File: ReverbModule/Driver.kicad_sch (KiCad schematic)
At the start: 29 parts, among them J1 Tank, J2 Screw_Terminal_01x02, Q1 BD139, Q2 BD140, U1 NE5532

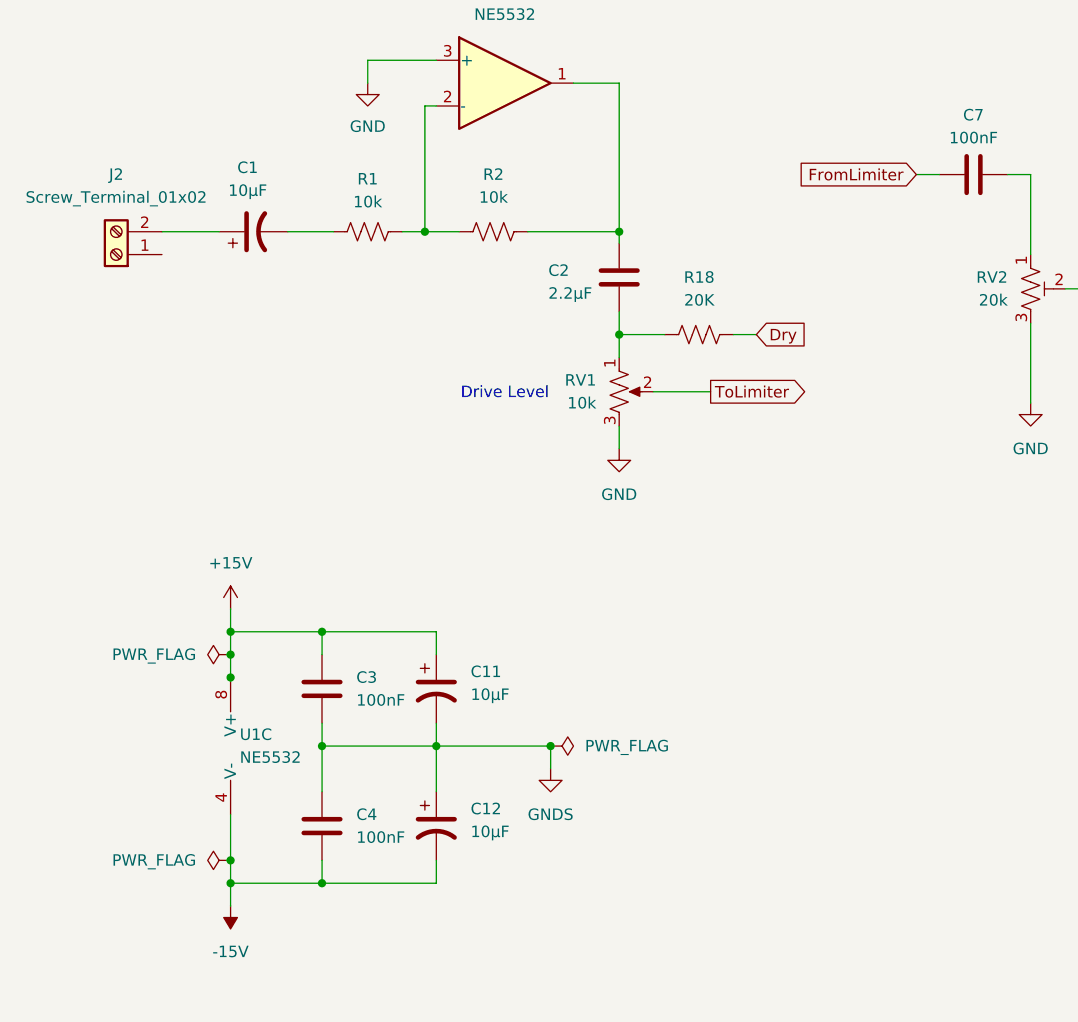
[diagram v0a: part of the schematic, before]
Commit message: Schematic Capture
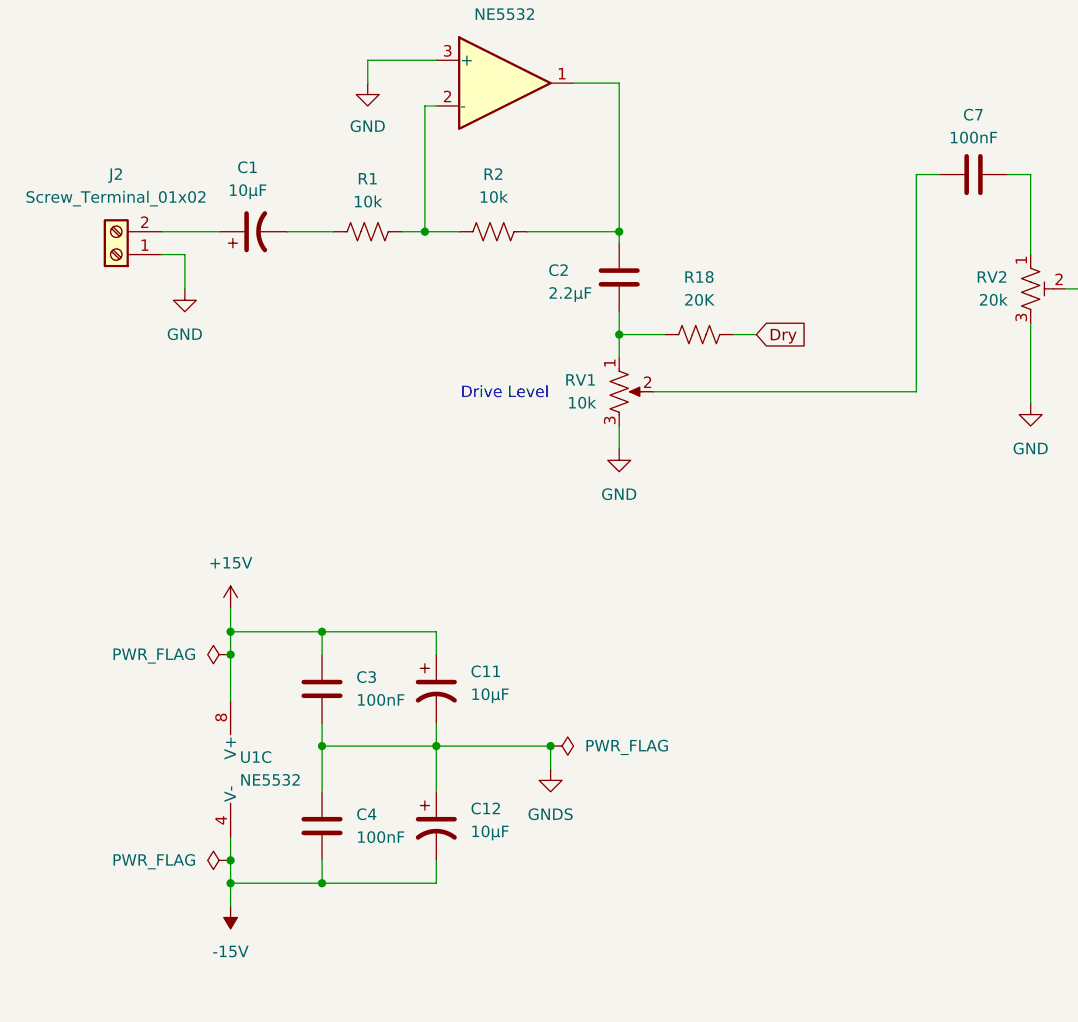
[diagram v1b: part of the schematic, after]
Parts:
- J2: footprint (none) -> TerminalBlock_Phoenix:TerminalBlock_Phoenix_MKDS-3-2-5.08_1x02_P5.08mm_Horizontal
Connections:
- net ToLimiter is gone; now on an unnamed net: RV1.2
- net GND: now also J2.1 (Pin_1)
- net FromLimiter: no longer names the net of C7.1
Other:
- moved on the sheet: U1C
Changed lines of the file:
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@@
 	)
 	(junction
-		(at 38.1 119.38)
+		(at 38.1 139.7)
 		(diameter 0)
 		(color 0 0 0 0)
@@
 	)
 	(junction
-		(at 200.66 63.5)
+		(at 38.1 116.84)
 		(diameter 0)
 		(color 0 0 0 0)
 	)
 	(junction
-		(at 203.2 88.9)
+		(at 200.66 63.5)
 		(diameter 0)
 		(color 0 0 0 0)
 	)
 	(junction
-		(at 38.1 142.24)
+		(at 203.2 88.9)
 		(diameter 0)
 		(color 0 0 0 0)
 	)
 	(junction
-		(at 38.1 116.84)
+		(at 38.1 142.24)
 		(diameter 0)
 		(color 0 0 0 0)
@@
 	)
 	(junction
-		(at 38.1 139.7)
-		(diameter 0)
-		(color 0 0 0 0)
-	)
-	(junction
 		(at 60.96 127)
 		(diameter 0)
@@
 	(wire
 		(pts
+			(xy 33.02 72.39) (xy 33.02 76.2)
+		)
+		(stroke
+			(width 0)
+			(type default)
+		)
+	)
+	(wire
+		(pts
+			(xy 114.3 63.5) (xy 114.3 87.63)
+		)
+		(stroke
+			(width 0)
+			(type default)
+		)
+	)
+	(wire
+		(pts
 			(xy 81.28 69.85) (xy 81.28 53.34)
 		)
@@
 	(wire
 		(pts
-			(xy 85.09 87.63) (xy 91.44 87.63)
+			(xy 85.09 87.63) (xy 114.3 87.63)
 		)
 		(stroke
@@
 	(wire
 		(pts
-			(xy 38.1 116.84) (xy 38.1 119.38)
+			(xy 53.34 50.8) (xy 53.34 53.34)
 		)
 		(stroke
@@
 	(wire
 		(pts
-			(xy 53.34 50.8) (xy 53.34 53.34)
+			(xy 144.78 86.36) (xy 144.78 88.9)
 		)
 		(stroke
@@
 	(wire
 		(pts
-			(xy 144.78 86.36) (xy 144.78 88.9)
+			(xy 44.45 69.85) (xy 49.53 69.85)
 		)
 		(stroke
@@
 	(wire
 		(pts
-			(xy 44.45 69.85) (xy 49.53 69.85)
+			(xy 60.96 127) (xy 73.66 127)
 		)
 		(stroke
@@
 	(wire
 		(pts
-			(xy 60.96 127) (xy 73.66 127)
+			(xy 185.42 60.96) (xy 185.42 63.5)
 		)
 		(stroke
@@
 	(wire
 		(pts
-			(xy 185.42 60.96) (xy 185.42 63.5)
+			(xy 152.4 104.14) (xy 152.4 77.47)
 		)
 		(stroke
@@
 	(wire
 		(pts
-			(xy 152.4 104.14) (xy 152.4 77.47)
+			(xy 38.1 137.16) (xy 38.1 139.7)
 		)
 		(stroke
@@
 	(wire
 		(pts
-			(xy 38.1 139.7) (xy 38.1 142.24)
+			(xy 81.28 53.34) (xy 76.2 53.34)
 		)
 		(stroke
@@
 	(wire
 		(pts
-			(xy 81.28 53.34) (xy 76.2 53.34)
+			(xy 38.1 116.84) (xy 38.1 121.92)
 		)
 		(stroke
@@
 	(wire
 		(pts
-			(xy 185.42 76.2) (xy 185.42 78.74)
+			(xy 30.48 72.39) (xy 33.02 72.39)
 		)
 		(stroke
@@
 	(wire
 		(pts
-			(xy 162.56 66.04) (xy 160.02 66.04)
+			(xy 185.42 76.2) (xy 185.42 78.74)
 		)
 		(stroke
@@
 	(wire
 		(pts
-			(xy 220.98 38.1) (xy 220.98 45.72)
+			(xy 162.56 66.04) (xy 160.02 66.04)
 		)
 		(stroke
@@
 	(wire
 		(pts
-			(xy 38.1 134.62) (xy 38.1 139.7)
+			(xy 220.98 38.1) (xy 220.98 45.72)
 		)
 		(stroke
@@
 	(wire
 		(pts
-			(xy 38.1 119.38) (xy 38.1 119.634)
-		)
-		(stroke
-			(width 0)
-			(type default)
-		)
-	)
-	(wire
-		(pts
 			(xy 38.1 111.76) (xy 38.1 114.3)
 		)
@@
 	(wire
 		(pts
+			(xy 38.1 139.7) (xy 38.1 142.24)
+		)
+		(stroke
+			(width 0)
+			(type default)
+		)
+	)
+	(wire
+		(pts
 			(xy 231.14 63.5) (xy 231.14 71.12)
 		)
@@
 		)
 	)
-	(global_label "ToLimiter"
-		(shape output)
-		(at 91.44 87.63 0)
-		(fields_autoplaced yes)
-		(effects
-			(font
-				(size 1.27 1.27)
-			)
-			(justify left)
-		)
-		(property "Intersheetrefs" "${INTERSHEET_REFS}"
-			(at 103.0733 87.63 0)
-			(hide yes)
-			(show_name no)
-			(do_not_autoplace no)
-			(effects
-				(font
-					(size 1.27 1.27)
-				)
-				(justify left)
-			)
-		)
-	)
-	(global_label "FromLimiter"
-		(shape input)
-		(at 114.3 63.5 180)
-		(fields_autoplaced yes)
-		(effects
-			(font
-				(size 1.27 1.27)
-			)
-			(justify right)
-		)
-		(property "Intersheetrefs" "${INTERSHEET_REFS}"
-			(at 100.0662 63.5 0)
-			(hide yes)
-			(show_name no)
-			(do_not_autoplace no)
-			(effects
-				(font
-					(size 1.27 1.27)
-				)
-				(justify right)
-			)
-		)
-	)
 	(global_label "Dry"
 		(shape input)
@@
 			)
 		)
-		(property "Footprint" ""
+		(property "Footprint" "TerminalBlock_Phoenix:TerminalBlock_Phoenix_MKDS-3-2-5.08_1x02_P5.08mm_Horizontal"
 			(at 25.4 72.39 0)
 			(hide yes)
@@
 	(symbol
 		(lib_id "Amplifier_Operational:NE5532")
-		(at 40.64 127 0)
+		(at 40.64 129.54 0)
 		(unit 3)
 		(body_style 1)
@@
 		(fields_autoplaced yes)
 		(property "Reference" "U1"
-			(at 39.116 125.7299 0)
+			(at 39.116 128.2699 0)
 			(show_name no)
 			(do_not_autoplace no)
@@
 		)
 		(property "Value" "NE5532"
-			(at 39.116 128.2699 0)
+			(at 39.116 130.8099 0)
 			(show_name no)
 			(do_not_autoplace no)
@@
 		)
 		(property "Footprint" "Package_SO:SOIC-8_3.9x4.9mm_P1.27mm"
-			(at 40.64 127 0)
+			(at 40.64 129.54 0)
 			(hide yes)
 			(show_name no)
@@
 		)
 		(property "Datasheet" "http://www.ti.com/lit/ds/symlink/ne5532.pdf"
-			(at 40.64 127 0)
+			(at 40.64 129.54 0)
 			(hide yes)
 			(show_name no)
@@
 		)
 		(property "Description" "Dual Low-Noise Operational Amplifiers, DIP-8/SOIC-8"
-			(at 40.64 127 0)
+			(at 40.64 129.54 0)
 			(hide yes)
 			(show_name no)
@@
 		)
 		(property "MPN" "NE5532DR"
-			(at 40.64 127 0)
+			(at 40.64 129.54 0)
 			(hide yes)
 			(show_name no)
@@
 		)
 		(property "LCSC" "C7426"
-			(at 40.64 127 0)
+			(at 40.64 129.54 0)
 			(hide yes)
 			(show_name no)
@@
 					(unit 1)
 				)
+			)
+		)
+	)
+	(symbol
+		(lib_id "power:GND")
+		(at 33.02 76.2 0)
+		(unit 1)
+		(body_style 1)
+		(exclude_from_sim no)
+		(in_bom yes)
+		(on_board yes)
+		(in_pos_files yes)
+		(dnp no)
+		(fields_autoplaced yes)
+		(property "Reference" "#PWR023"
+			(at 33.02 82.55 0)
+			(hide yes)
+			(show_name no)
+			(do_not_autoplace no)
+			(effects
+				(font
+					(size 1.27 1.27)
+				)
+			)
+		)
+		(property "Value" "GND"
+			(at 33.02 81.28 0)
+			(show_name no)
+			(do_not_autoplace no)
+			(effects
+				(font
+					(size 1.27 1.27)
+				)
+			)
+		)
+		(property "Footprint" ""
+			(at 33.02 76.2 0)
+			(hide yes)
+			(show_name no)
+			(do_not_autoplace no)
+			(effects
+				(font
+					(size 1.27 1.27)
+				)
+			)
+		)
+		(property "Datasheet" ""
+			(at 33.02 76.2 0)
+			(hide yes)
+			(show_name no)
+			(do_not_autoplace no)
+			(effects
+				(font
+					(size 1.27 1.27)
+				)
+			)
+		)
+		(property "Description" "Power symbol creates a global label with name \"GND\" , ground"
+			(at 33.02 76.2 0)
+			(hide yes)
+			(show_name no)
+			(do_not_autoplace no)
+			(effects
+				(font
+					(size 1.27 1.27)
+				)
+			)
+		)
+		(pin "1"
+		)
+		(instances
+			(project "ReverbModule"
+				(path "/e19e1d15-f0b3-4286-a818-bc907405212b/c6d45d4c-e85e-4a36-afcc-7c11e84777bd"
+					(reference "#PWR023")
+					(unit 1)
+				)
